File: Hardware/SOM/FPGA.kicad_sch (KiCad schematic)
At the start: 19 parts, among them U1 LFE5UM5G-85F

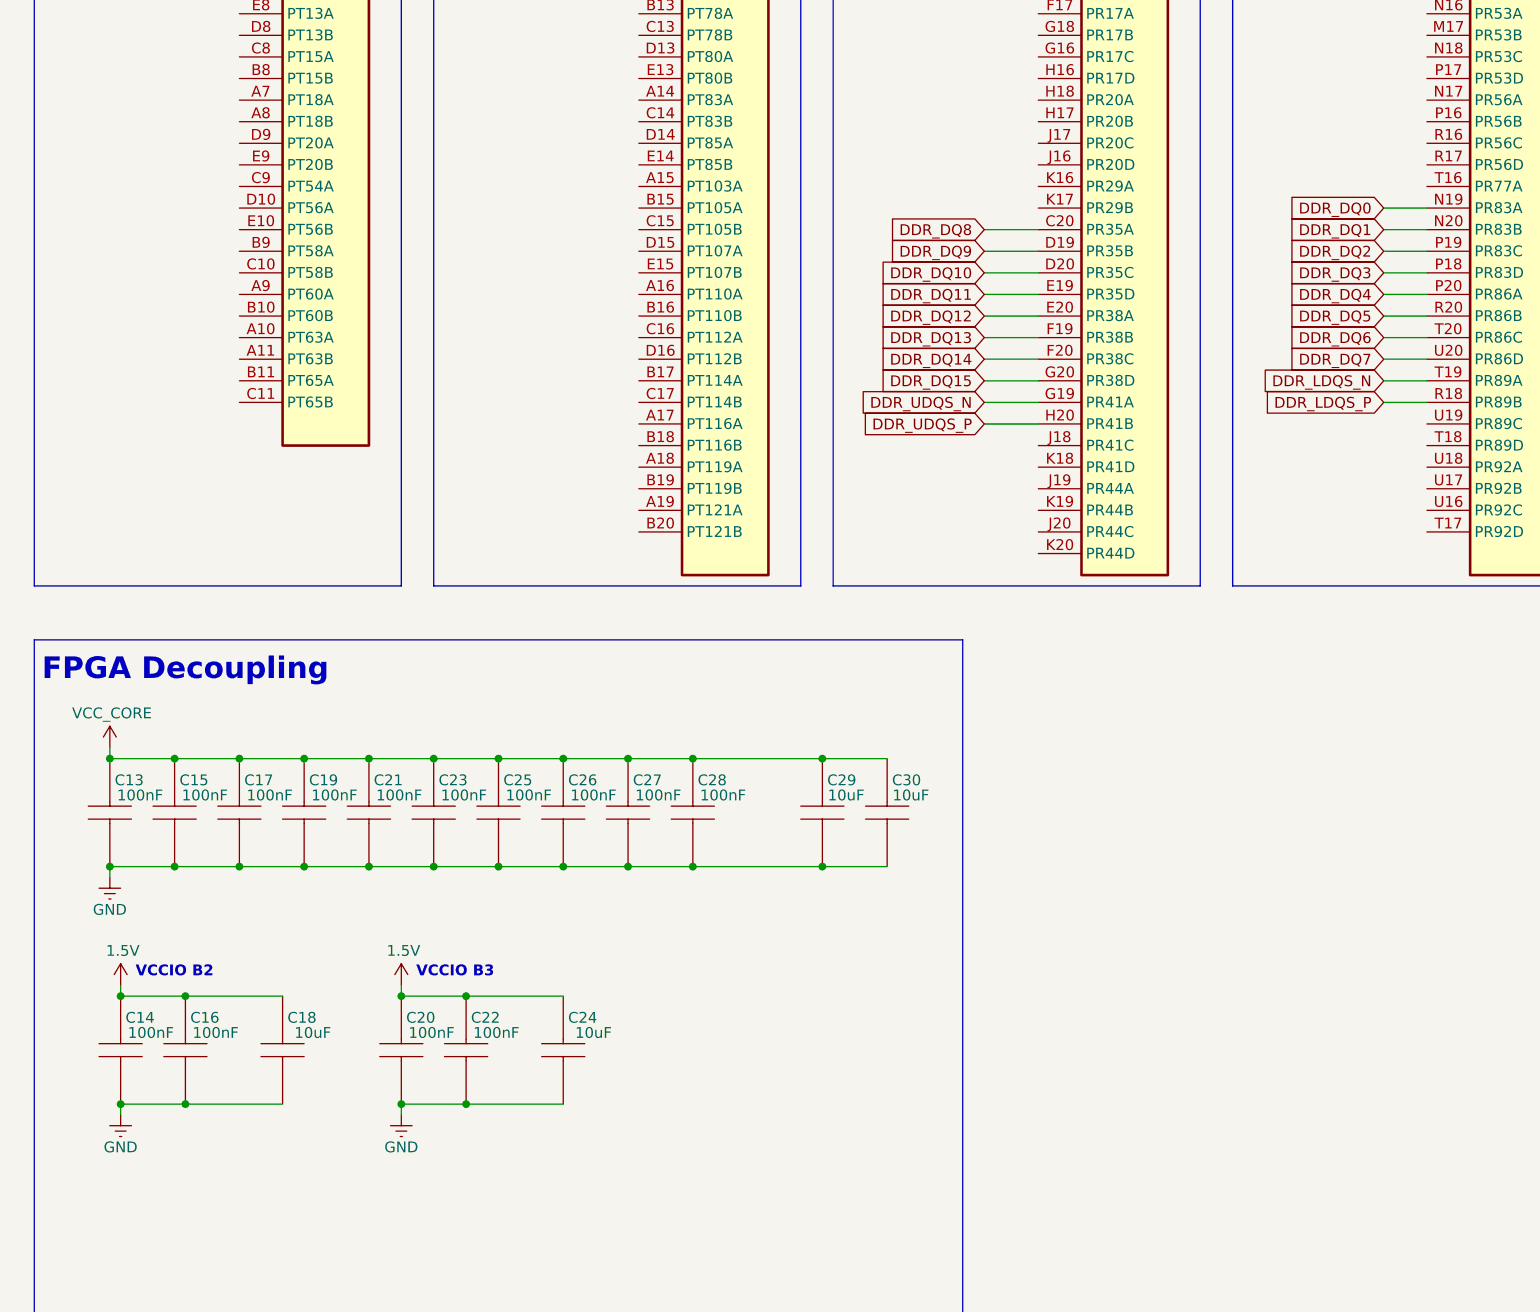
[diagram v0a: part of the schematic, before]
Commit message: some schematics update
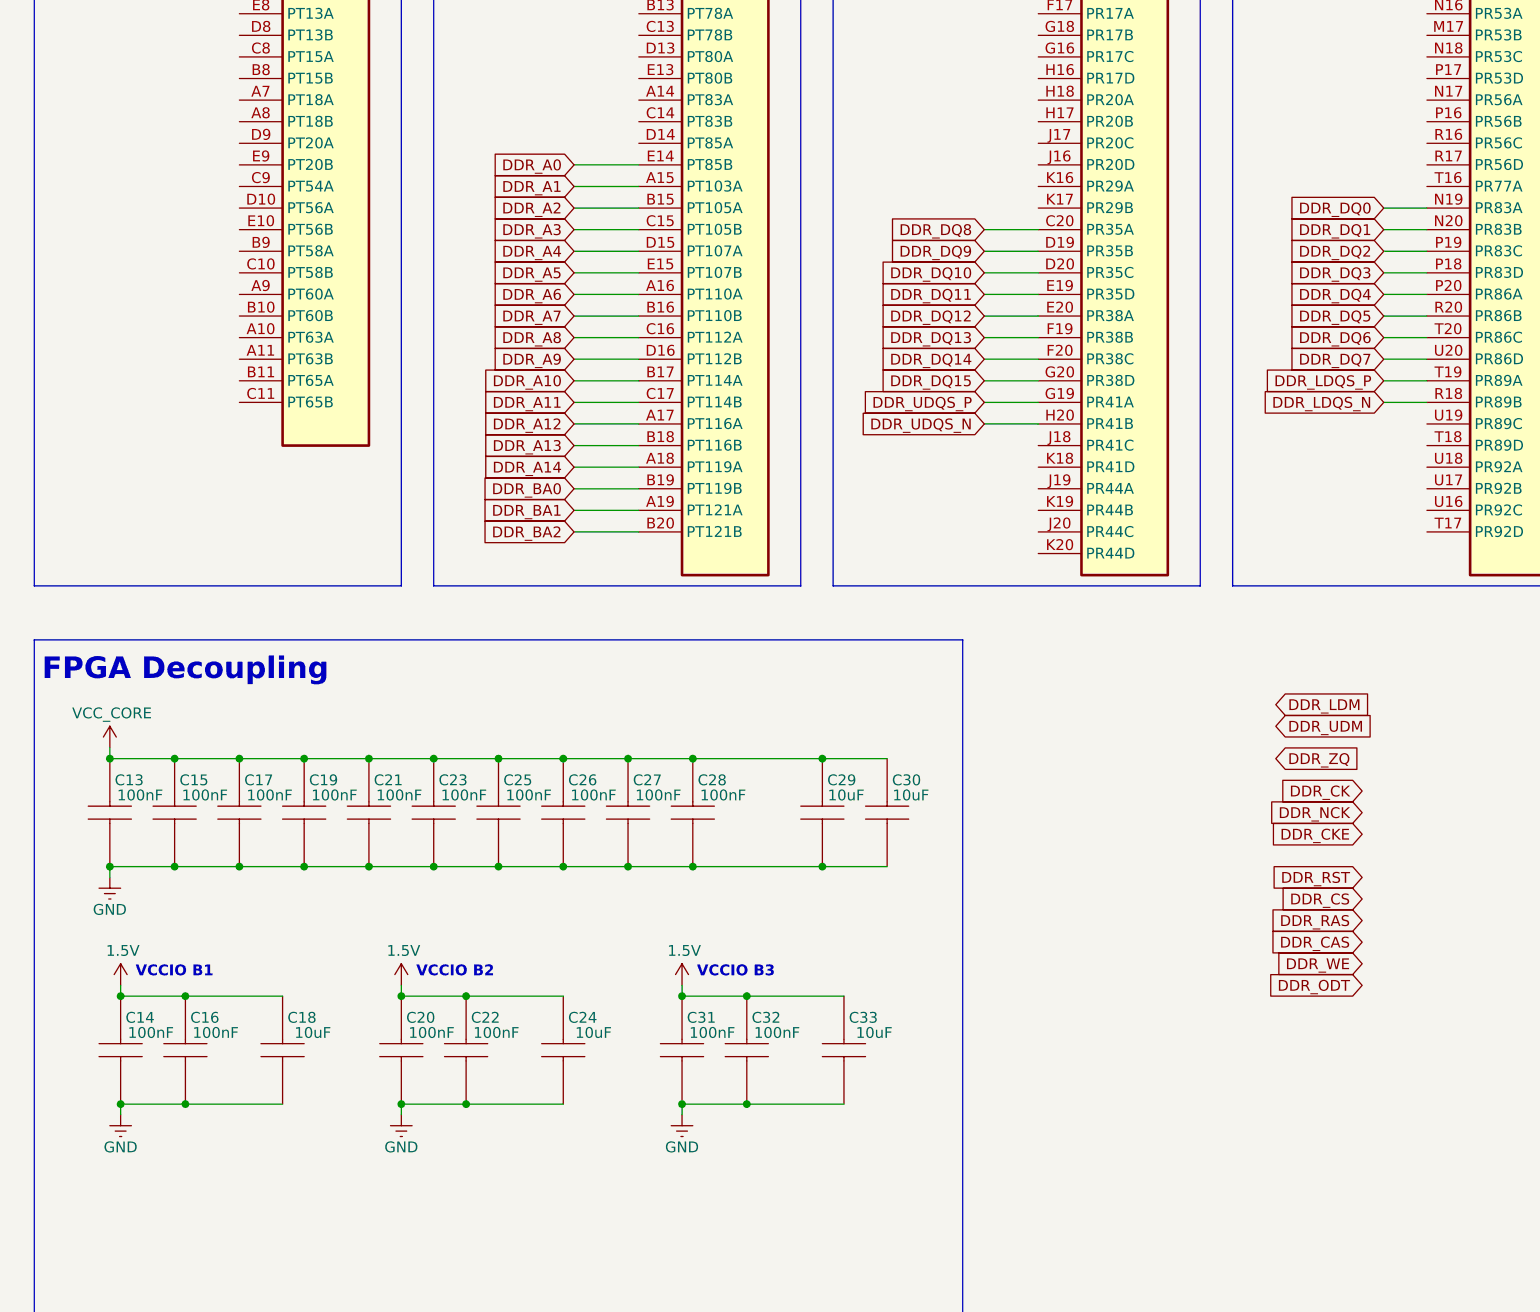
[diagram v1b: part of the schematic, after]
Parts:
- added C31, C32: 100nF, Capacitor_SMD:C_0402_1005Metric, symbol RA8M1:885012205092
- added C33: 10uF, Capacitor_SMD:C_0402_1005Metric, symbol RA8M1:885012205092
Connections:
- net 1.5V: now also C31.2, C32.2, C33.2
- net DDR_LDQS_N: now also U1.R18 (PR89B); no longer U1.T19 (PR89A)
- net DDR_LDQS_P: now also U1.T19 (PR89A); no longer U1.R18 (PR89B)
- net DDR_UDQS_N: now also U1.H20 (PR41B); no longer U1.G19 (PR41A)
- net DDR_UDQS_P: now also U1.G19 (PR41A); no longer U1.H20 (PR41B)
- net GND: now also C31.1, C32.1, C33.1
- net DDR_A1: now reaches U1.A15 (PT103A)
- net DDR_A6: now reaches U1.A16 (PT110A)
- net DDR_A12: now reaches U1.A17 (PT116A)
- net DDR_A14: now reaches U1.A18 (PT119A)
- net DDR_BA1: now reaches U1.A19 (PT121A)
- net DDR_A2: now reaches U1.B15 (PT105A)
- net DDR_A7: now reaches U1.B16 (PT110B)
- net DDR_A10: now reaches U1.B17 (PT114A)
- net DDR_A13: now reaches U1.B18 (PT116B)
- net DDR_BA0: now reaches U1.B19 (PT119B)
- net DDR_BA2: now reaches U1.B20 (PT121B)
- net DDR_A3: now reaches U1.C15 (PT105B)
- net DDR_A8: now reaches U1.C16 (PT112A)
- net DDR_A11: now reaches U1.C17 (PT114B)
- net DDR_A4: now reaches U1.D15 (PT107A)
- net DDR_A9: now reaches U1.D16 (PT112B)
- net DDR_A0: now reaches U1.E14 (PT85B)
- net DDR_A5: now reaches U1.E15 (PT107B)
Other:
- note added: "VCCIO B1"
